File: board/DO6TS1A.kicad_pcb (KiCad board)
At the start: 2 copper layers, 60 x 55 mm, 36 parts, among them U1 PCF8574, U2 RT9193, U3 HLK-PM01, U4 ESP-12, U5 LTV-354T, X1 ESP-PROG

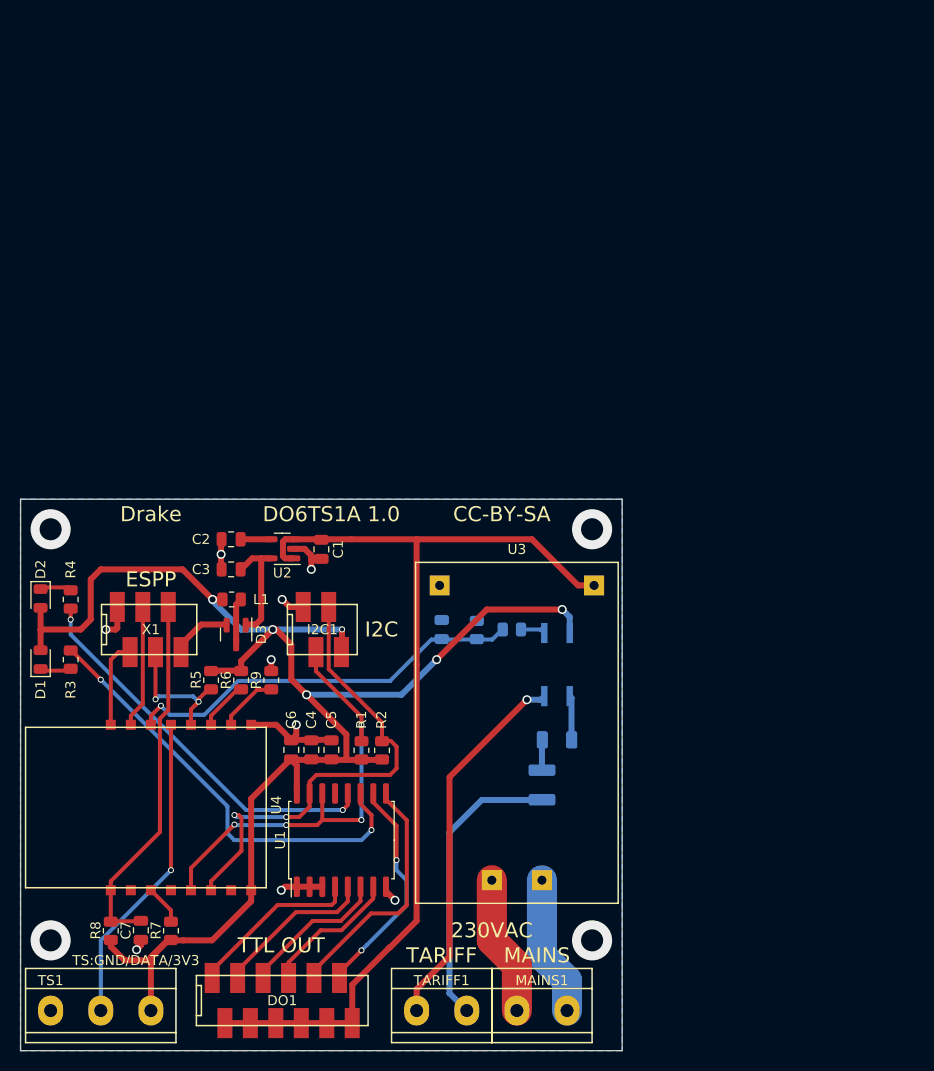
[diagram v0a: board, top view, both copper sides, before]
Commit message: WIP
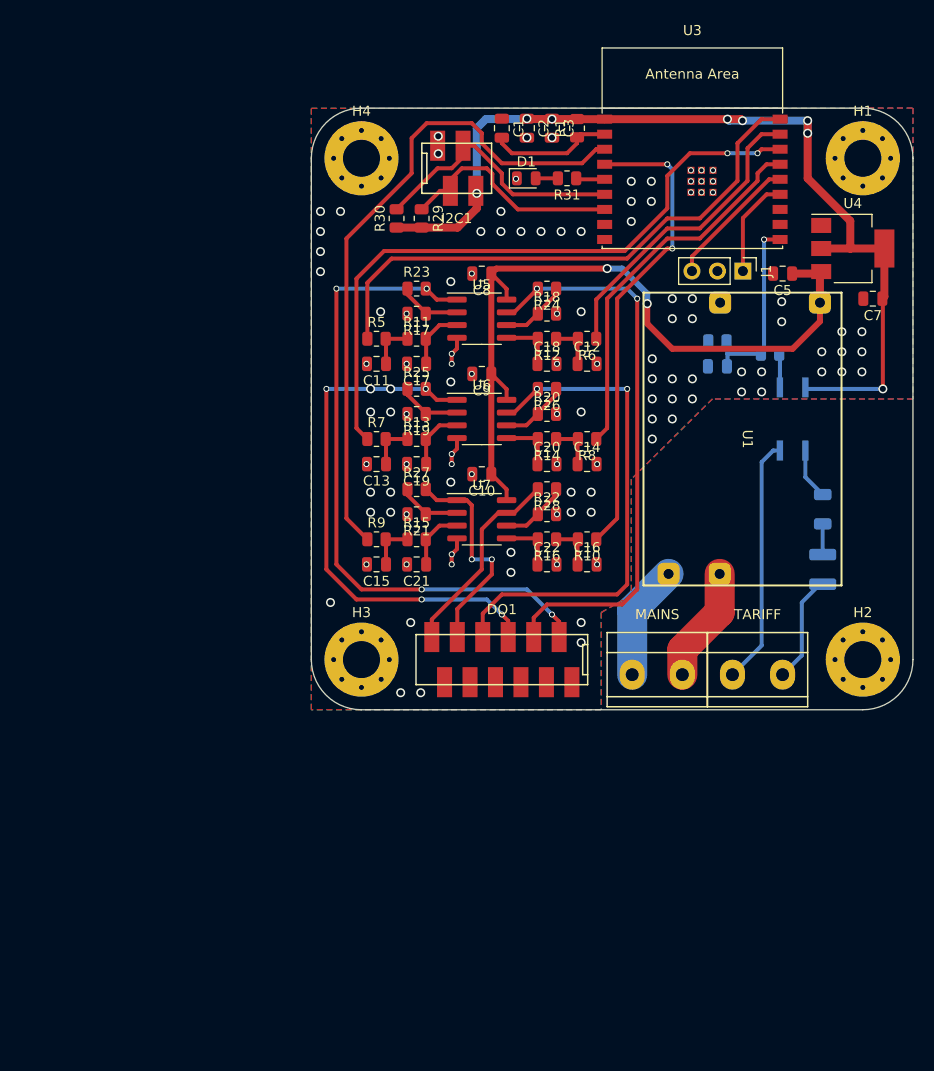
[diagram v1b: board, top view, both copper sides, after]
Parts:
- removed D2: LED, LED_SMD:LED_0805_2012Metric
- removed D3: BAT54C, Package_TO_SOT_SMD:SOT-23
- removed L1: Ferrite bead, Resistor_SMD:R_0805_2012Metric
- removed MAINS1, TARIFF1: Conn_01x02, Drake:DG301-5.0-02
- removed TS1: Conn_01x03, Drake:DG301-5.0-03
- added C10: 100n, Capacitor_SMD:C_0805_2012Metric, F.Cu at (126.0, 82.5)
- added C11: 100n, Capacitor_SMD:C_0805_2012Metric, F.Cu at (115.5, 71.5)
- added C12: 100n, Capacitor_SMD:C_0805_2012Metric, F.Cu at (136.5, 71.5)
- added C13: 100n, Capacitor_SMD:C_0805_2012Metric, F.Cu at (115.5, 81.5)
- added C14: 100n, Capacitor_SMD:C_0805_2012Metric, F.Cu at (136.5, 81.5)
- added C15: 100n, Capacitor_SMD:C_0805_2012Metric, F.Cu at (115.5, 91.5)
- added C16: 100n, Capacitor_SMD:C_0805_2012Metric, F.Cu at (136.5, 91.5)
- added C17: 100n, Capacitor_SMD:C_0805_2012Metric, F.Cu at (119.5, 71.5)
- added C18: 100n, Capacitor_SMD:C_0805_2012Metric, F.Cu at (132.5, 71.5)
- added C19: 100n, Capacitor_SMD:C_0805_2012Metric, F.Cu at (119.5, 81.5)
- added C20: 100n, Capacitor_SMD:C_0805_2012Metric, F.Cu at (132.5, 81.5)
- added C21: 100n, Capacitor_SMD:C_0805_2012Metric, F.Cu at (119.5, 91.5)
- added C22: 100n, Capacitor_SMD:C_0805_2012Metric, F.Cu at (132.5, 91.5)
- added H1: MountingHole, MountingHole:MountingHole_3.7mm_Pad_Via, F.Cu at (164.0, 51.0)
- added H2: MountingHole, MountingHole:MountingHole_3.7mm_Pad_Via, F.Cu at (164.0, 101.0)
- added H3: MountingHole, MountingHole:MountingHole_3.7mm_Pad_Via, F.Cu at (114.0, 101.0)
- added H4: MountingHole, MountingHole:MountingHole_3.7mm_Pad_Via, F.Cu at (114.0, 51.0)
- added J1: PROG, Connector_PinHeader_2.54mm:PinHeader_1x03_P2.54mm_Vertical, F.Cu at (152.0, 62.2)
- added R13: 1k5, Resistor_SMD:R_0805_2012Metric, F.Cu at (119.5, 79.0)
- added R14: 1k5, Resistor_SMD:R_0805_2012Metric, F.Cu at (132.5, 79.0)
- added R15: 1k5, Resistor_SMD:R_0805_2012Metric, F.Cu at (119.5, 89.0)
- added R16: 1k5, Resistor_SMD:R_0805_2012Metric, F.Cu at (132.5, 89.0)
- added R17: 100k, Resistor_SMD:R_0805_2012Metric, F.Cu at (119.5, 66.5)
- added R18: 100k, Resistor_SMD:R_0805_2012Metric, F.Cu at (132.5, 66.5)
- added R19: 100k, Resistor_SMD:R_0805_2012Metric, F.Cu at (119.5, 76.5)
- added R20: 100k, Resistor_SMD:R_0805_2012Metric, F.Cu at (132.5, 76.5)
- added R21: 100k, Resistor_SMD:R_0805_2012Metric, F.Cu at (119.5, 86.5)
- added R22: 100k, Resistor_SMD:R_0805_2012Metric, F.Cu at (132.5, 86.5)
- added R23: 56k, Resistor_SMD:R_0805_2012Metric, F.Cu at (119.5, 64.0)
- added R24: 56k, Resistor_SMD:R_0805_2012Metric, F.Cu at (132.5, 64.0)
- added R25: 56k, Resistor_SMD:R_0805_2012Metric, F.Cu at (119.5, 74.0)
- added R26: 56k, Resistor_SMD:R_0805_2012Metric, F.Cu at (132.5, 74.0)
- added R27: 56k, Resistor_SMD:R_0805_2012Metric, F.Cu at (119.5, 84.0)
- added R28: 56k, Resistor_SMD:R_0805_2012Metric, F.Cu at (132.5, 84.0)
- added R29: 10k, Resistor_SMD:R_0805_2012Metric, F.Cu at (120.0, 57.0)
- added R30: 10k, Resistor_SMD:R_0805_2012Metric, F.Cu at (117.5, 57.0)
- added R31: 270R, Resistor_SMD:R_0805_2012Metric, F.Cu at (134.5, 53.0)
- added U6: LM358, Package_SO:SOIC-8_3.9x4.9mm_P1.27mm, F.Cu at (126.0, 77.0)
- added U7: LM358, Package_SO:SOIC-8_3.9x4.9mm_P1.27mm, F.Cu at (126.0, 87.0)
- added X2: TARIFF, Drake:DG301-5.0-02, F.Cu at (151.0, 102.5)
- C2: value 22n -> 47u
- C3: value 1u -> 47u
- C4: value 47u -> 100n; footprint Capacitor_SMD:C_0805_2012Metric -> Capacitor_SMD:C_1210_3225Metric; moved to B.Cu
- C5: value 47u -> 10u
- C6: value 100n -> 1u; moved to B.Cu
- C7: value 100n -> 10u
- C8: footprint Capacitor_SMD:C_1210_3225Metric -> Capacitor_SMD:C_0805_2012Metric; moved to F.Cu
- C9: value 1u -> 100n; moved to F.Cu
- DO1: value Conn_02x06_Odd_Even -> Regulators
- R10: footprint Resistor_SMD:R_1206_3216Metric -> Resistor_SMD:R_0805_2012Metric; moved to F.Cu
- R11: moved to F.Cu
- R12: value 56k -> 1k5; moved to F.Cu
- R2: value 10k -> 1k5; footprint Resistor_SMD:R_0805_2012Metric -> Resistor_SMD:R_1206_3216Metric; moved to B.Cu
- R3: value 270R -> 1k5; moved to B.Cu
- R4: value 270R -> 56k; moved to B.Cu
- R5, R6, R7, R8, R9: value 10k -> 1k5
- U1: value PCF8574 -> YS-12V450A; footprint Package_SO:SOIC-16W_7.5x10.3mm_P1.27mm -> Drake:YS-12V450A
- U2: value RT9193 -> LTV-354T; footprint Package_TO_SOT_SMD:SOT-23-5 -> Package_SO:SO-4_4.4x3.6mm_P2.54mm; moved to B.Cu
- U3: value HLK-PM01 -> ESP32-C3-WROOM-02; footprint Drake:HLK-PM01 -> Espressif:ESP32-C3-WROOM-02
- U4: value ESP-12 -> LM1117MP-3.3; footprint Drake:ESP-12 -> Package_TO_SOT_SMD:SOT-223-3_TabPin2
- U5: value LTV-354T -> LM358; footprint Package_SO:SO-4_4.4x3.6mm_P2.54mm -> Package_SO:SOIC-8_3.9x4.9mm_P1.27mm; moved to F.Cu
- X1: value ESP-PROG -> MAINS; footprint Drake:Micro-Match-FOB-6 -> Drake:DG301-5.0-02
- moved C7 96.4 mm to (165.0, 65.0), turned to 180 degrees
- moved U4 80.8 mm to (163.0, 60.0), turned to 0 degrees
- moved R3 76.1 mm to (154.8, 70.5), turned to 180 degrees
- moved R4 69.5 mm to (149.5, 69.2), turned to 180 degrees
- moved R8 68.3 mm to (136.5, 79.0), turned to 180 degrees
- moved D1 68.2 mm to (130.4, 53.0), turned to 0 degrees
- moved R1 65.7 mm to (135.5, 48.0), turned to 90 degrees
- moved C5 65.4 mm to (156.0, 62.5), turned to 180 degrees
- moved U3 59.7 mm to (147.0, 51.2), turned to 0 degrees
- moved C6 57.2 mm to (149.5, 71.8), turned to 0 degrees
- moved U1 56.6 mm to (152.0, 79.0), turned to -90 degrees
- moved C3 54.4 mm to (133.0, 48.0), turned to -90 degrees
- moved C4 54.1 mm to (160.0, 92.0), turned to -90 degrees
- moved R7 53.2 mm to (115.5, 79.0), turned to 0 degrees
- moved U2 52.5 mm to (157.0, 77.0), turned to 90 degrees
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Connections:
- C1 pad 1: /5V -> GND
- C1 pad 2: GND -> Net-(U3-EN/CHIP_PU)
- C2 pad 1: Net-(C2-Pad1) -> +3V3
- C3 pad 1: Net-(C3-Pad1) -> +3V3
- C4 pad 1: VCC -> Net-(C4-Pad1)
- C4 pad 2: GND -> Net-(X2-Pin_2)
- C5 pad 1: VCC -> +12V
- C6 pad 1: VCC -> GND
- C6 pad 2: GND -> /TARIFF
- C7 pad 1: GND -> +3V3
- C7 pad 2: /ESP/RESET -> GND
- C8 pad 1: Net-(C8-Pad1) -> +12V
- C8 pad 2: Net-(C8-Pad2) -> GND
- C9 pad 1: GND -> +12V
- C9 pad 2: /TARIFF -> GND
- D1 pad 1: Net-(D1-Pad1) -> GND
- D1 pad 2: VCC -> Net-(D1-A)
- DO1 pad 1: Net-(DO1-Pad1) -> GND
- DO1 pad 10: /5V -> /AOUT4
- DO1 pad 11: Net-(DO1-Pad11) -> GND
- DO1 pad 12: /5V -> /AOUT5
- DO1 pad 2: /5V -> /AOUT0
- DO1 pad 3: Net-(DO1-Pad3) -> GND
- DO1 pad 4: /5V -> /AOUT1
- DO1 pad 5: Net-(DO1-Pad5) -> GND
- DO1 pad 6: /5V -> /AOUT2
- DO1 pad 7: Net-(DO1-Pad7) -> GND
- DO1 pad 8: /5V -> /AOUT3
- DO1 pad 9: Net-(DO1-Pad9) -> GND
- I2C1 pad 4: VCC -> +3V3
- R1 pad 1: /SCL -> Net-(U3-EN/CHIP_PU)
- R1 pad 2: VCC -> +3V3
- R10 pad 1: Net-(R10-Pad1) -> /DOUT5
- R10 pad 2: Net-(C8-Pad1) -> Net-(C16-Pad1)
- R11 pad 1: Net-(R11-Pad1) -> Net-(C11-Pad1)
- R11 pad 2: /TARIFF -> Net-(U5A-+)
- R12 pad 1: /TARIFF -> Net-(C12-Pad1)
- R12 pad 2: GND -> Net-(U5B-+)
- R2 pad 1: VCC -> Net-(R2-Pad1)
- R2 pad 2: /SDA -> Net-(C4-Pad1)
- R3 pad 2: Net-(D1-Pad1) -> /TARIFF
- R4 pad 1: Net-(R4-Pad1) -> /TARIFF
- R4 pad 2: Net-(D2-Pad1) -> GND
- R5 pad 1: /ESP/GPIO0 -> /DOUT0
- R5 pad 2: VCC -> Net-(C11-Pad1)
- R6 pad 1: /ESP/GPIO2 -> /DOUT1
- R6 pad 2: VCC -> Net-(C12-Pad1)
- R7 pad 1: /ESP/EN -> /DOUT2
- R7 pad 2: VCC -> Net-(C13-Pad1)
- R8 pad 1: /ESP/RESET -> /DOUT3
- R8 pad 2: VCC -> Net-(C14-Pad1)
- R9 pad 1: /ESP/GPIO15 -> /DOUT4
- R9 pad 2: GND -> Net-(C15-Pad1)
- U1 pad 1: GND -> Net-(U1-LINE1)
- U1 pad 2: GND -> Net-(U1-LINE2)
- U1 pad 4: Net-(DO1-Pad1) -> +12V
- U2 pad 1: /5V -> Net-(R2-Pad1)
- U2 pad 2: GND -> Net-(X2-Pin_1)
- U2 pad 3: /5V -> Net-(R3-Pad1)
- U2 pad 4: Net-(C2-Pad1) -> +3V3
- U3 pad 1: /ESP/MAINS-2 -> +3V3
- U3 pad 2: /ESP/MAINS-1 -> Net-(U3-EN/CHIP_PU)
- U3 pad 3: GND -> /DOUT4
- U3 pad 4: /5V -> /DOUT5
- U4 pad 1: /ESP/RESET -> GND
- U4 pad 2: /ESP/ADC -> +3V3
- U4 pad 3: /ESP/EN -> +12V
- U5 pad 1: Net-(R10-Pad1) -> /AOUT0
- U5 pad 3: Net-(R11-Pad1) -> Net-(U5A-+)
- U5 pad 4: VCC -> GND
- X1 pad 1: GND -> Net-(U1-LINE2)
- X1 pad 2: /ESP/TX -> Net-(U1-LINE1)
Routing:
- net VCC: track 154.7 -> 0.00 mm, vias 6 -> 0
- net /5V: track 99.2 -> 0.00 mm
- net +3V3: track 0.00 -> 98.3 mm, vias 0 -> 8
- net +12V: track 0.00 -> 76.9 mm, vias 0 -> 2
- net /DOUT4: track 0.00 -> 66.3 mm
- net /AOUT0: track 0.00 -> 66.2 mm, vias 0 -> 4
- net /DOUT2: track 0.00 -> 65.9 mm, vias 0 -> 2
- net /AOUT1: track 0.00 -> 56.9 mm, vias 0 -> 2
- net /DOUT0: track 0.00 -> 55.7 mm
- net /AOUT2: track 0.00 -> 53.4 mm, vias 0 -> 6
- net /AOUT3: track 0.00 -> 50.5 mm, vias 0 -> 2
- net /DOUT5: track 0.00 -> 47.3 mm, vias 0 -> 2
- net Net-(R3-Pad1): track 44.0 -> 3.38 mm, vias 2 -> 0
- net Net-(R4-Pad1): track 38.8 -> 0.00 mm, vias 2 -> 0
- net /DOUT3: track 0.00 -> 37.7 mm
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- added copper zone on F.Cu, net GND
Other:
- board size 60 x 55 mm -> 60 x 60 mm
- board text removed: "230VAC"
- board text removed: "Address:"
- board text removed: "CC-BY-SA"
- board text removed: "DO6TS1A 1.0"
- board text removed: "Drake"
- board text removed: "ESPP"
- board text removed: "I2C"
- board text removed: "MAINS"
- board text removed: "TARIFF"
- board text removed: "TS:GND/DATA/3V3"
- board text removed: "TTL OUT"
